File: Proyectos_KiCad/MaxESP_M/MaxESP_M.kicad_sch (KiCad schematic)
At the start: 0 parts

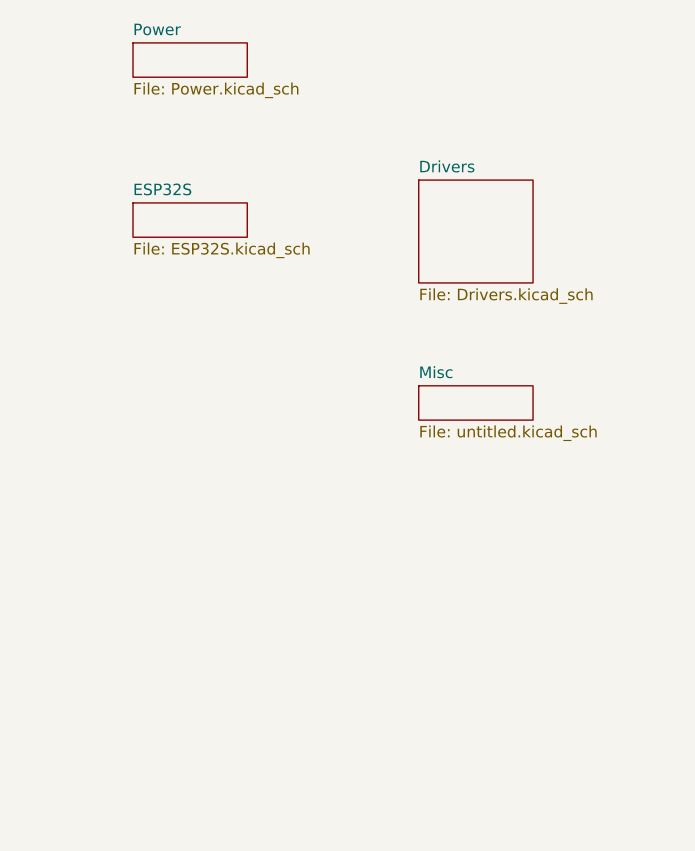
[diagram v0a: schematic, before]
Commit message: Por si valgo
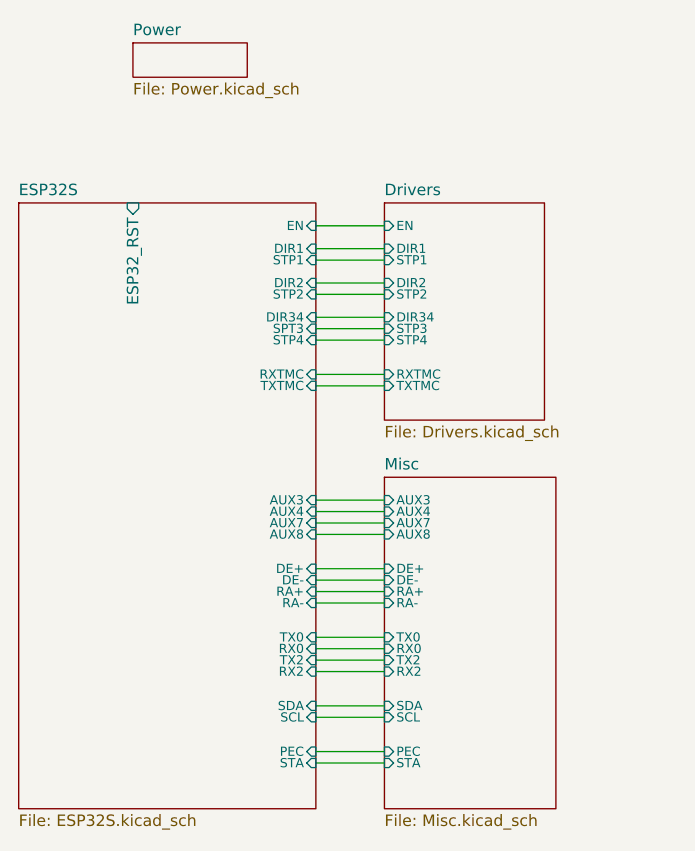
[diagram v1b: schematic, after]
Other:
- sheet Drivers ports: added DIR1, DIR2, DIR34, EN, RXTMC, STP1, STP2, STP3, STP4, TXTMC; removed none
- sheet ESP32S ports: added AUX3, AUX4, AUX7, AUX8, DE+, DE-, DIR1, DIR2, DIR34, EN, ESP32_RST, PEC, RA+, RA-, RX0, RX2, RXTMC, SCL, SDA, SPT3, STA, STP1, STP2, STP4, TX0, TX2, TXTMC; removed none
- sheet Misc: file untitled.kicad_sch -> Misc.kicad_sch
- sheet Misc ports: added AUX3, AUX4, AUX7, AUX8, DE+, DE-, PEC, RA+, RA-, RX0, RX2, SCL, SDA, STA, TX0, TX2; removed none
